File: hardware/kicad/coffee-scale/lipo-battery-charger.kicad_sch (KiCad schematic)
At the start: 9 parts, among them J1 JS2, U4 MCP73831-2-MC

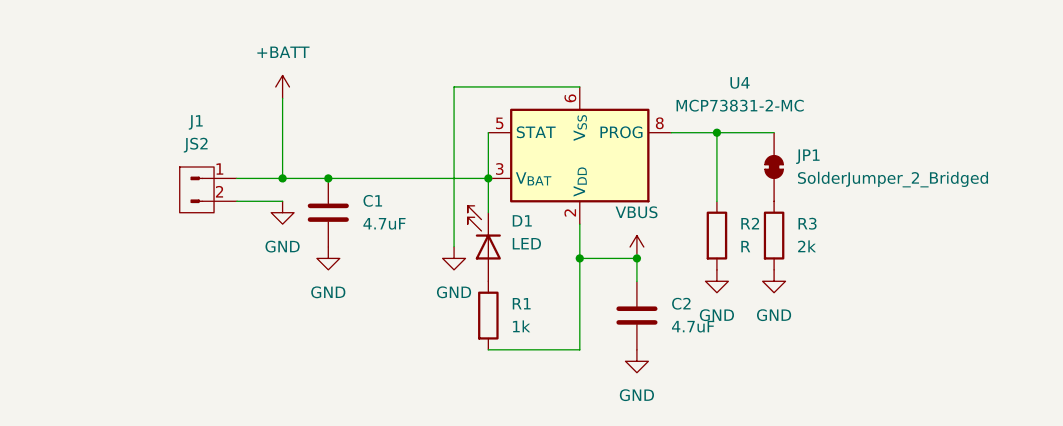
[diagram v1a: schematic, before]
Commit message: Update lipo-battery-charger.kicad_sch
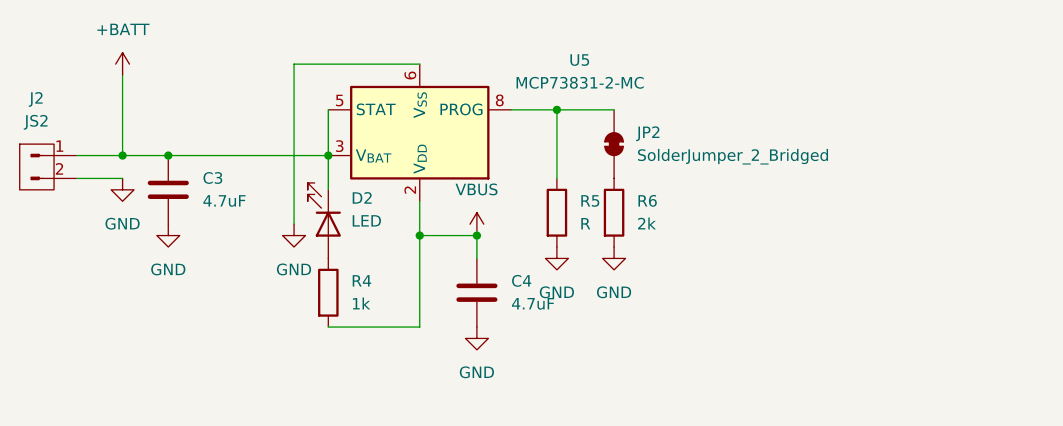
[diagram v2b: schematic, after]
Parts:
- removed C1, C2: 4.7uF, symbol Device:C
- removed D1: LED, symbol Device:LED
- removed J1: JS2, symbol Connector:Conn_01x02_Pin
- removed JP1: SolderJumper_2_Bridged, symbol Jumper:SolderJumper_2_Bridged
- removed R1: 1k, symbol Device:R
- removed R2: R, symbol Device:R
- removed R3: 2k, symbol Device:R
- removed U4: MCP73831-2-MC, Package_DFN_QFN:DFN-8-1EP_3x2mm_P0.5mm_EP1.7x1.4mm, symbol Battery_Management:MCP73831-2-MC
- added C3, C4: 4.7uF, symbol Device:C
- added D2: LED, symbol Device:LED
- added J2: JS2, symbol Connector:Conn_01x02_Pin
- added JP2: SolderJumper_2_Bridged, symbol Jumper:SolderJumper_2_Bridged
- added R4: 1k, symbol Device:R
- added R5: R, symbol Device:R
- added R6: 2k, symbol Device:R
- added U5: MCP73831-2-MC, Package_DFN_QFN:DFN-8-1EP_3x2mm_P0.5mm_EP1.7x1.4mm, symbol Battery_Management:MCP73831-2-MC
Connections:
- net +BATT: now also C3.1, D2.1 (K), J2.1 (Pin_1), U5.3 (V_{BAT}), U5.4 (V_{BAT}), U5.5 (STAT)
- net GND: now also C3.2, C4.2, J2.2 (Pin_2), R5.2, R6.2, U5.6 (V_{SS})
- net VBUS: now also C4.1, R4.2, U5.1 (V_{DD}), U5.2 (V_{DD})
- new net: D2.2 (A), R4.1
- new net: JP2.1 (A), R6.1
- new net: JP2.2 (B), R5.1, U5.8 (PROG)
